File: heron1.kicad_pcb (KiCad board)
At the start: 2 copper layers, 38 parts, among them J1 7.4 V BAT, J2 Conn_02x11_Counter_Clockwise, J3 MotorA, J4 Motor B, SW1 SW_Wuerth_450301014042, U1 ESP32-S3-DevKitC, U2 L7805, U4 L7806, U6 VNH5019A-E, U7 VNH5019A-E

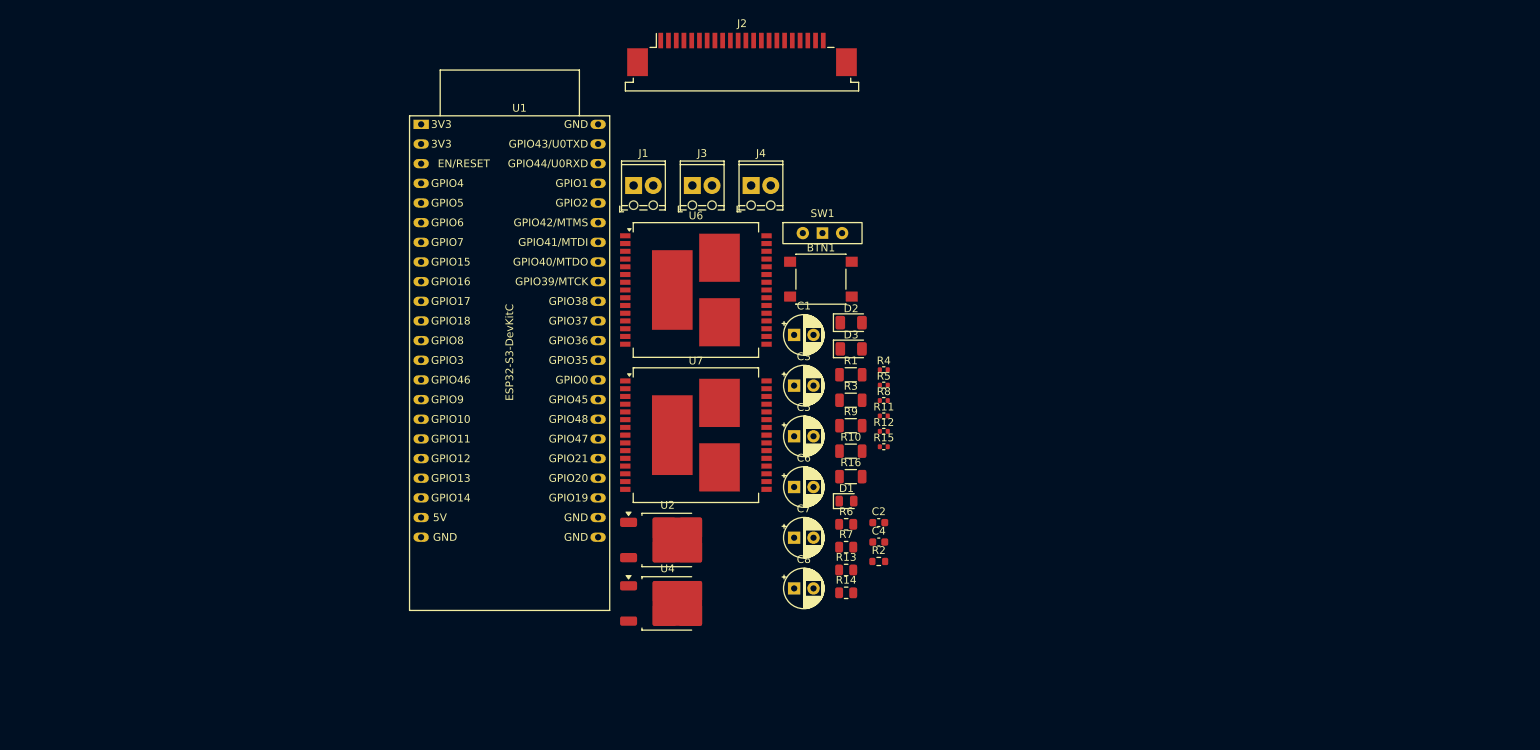
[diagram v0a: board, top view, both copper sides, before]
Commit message: first stage pcb
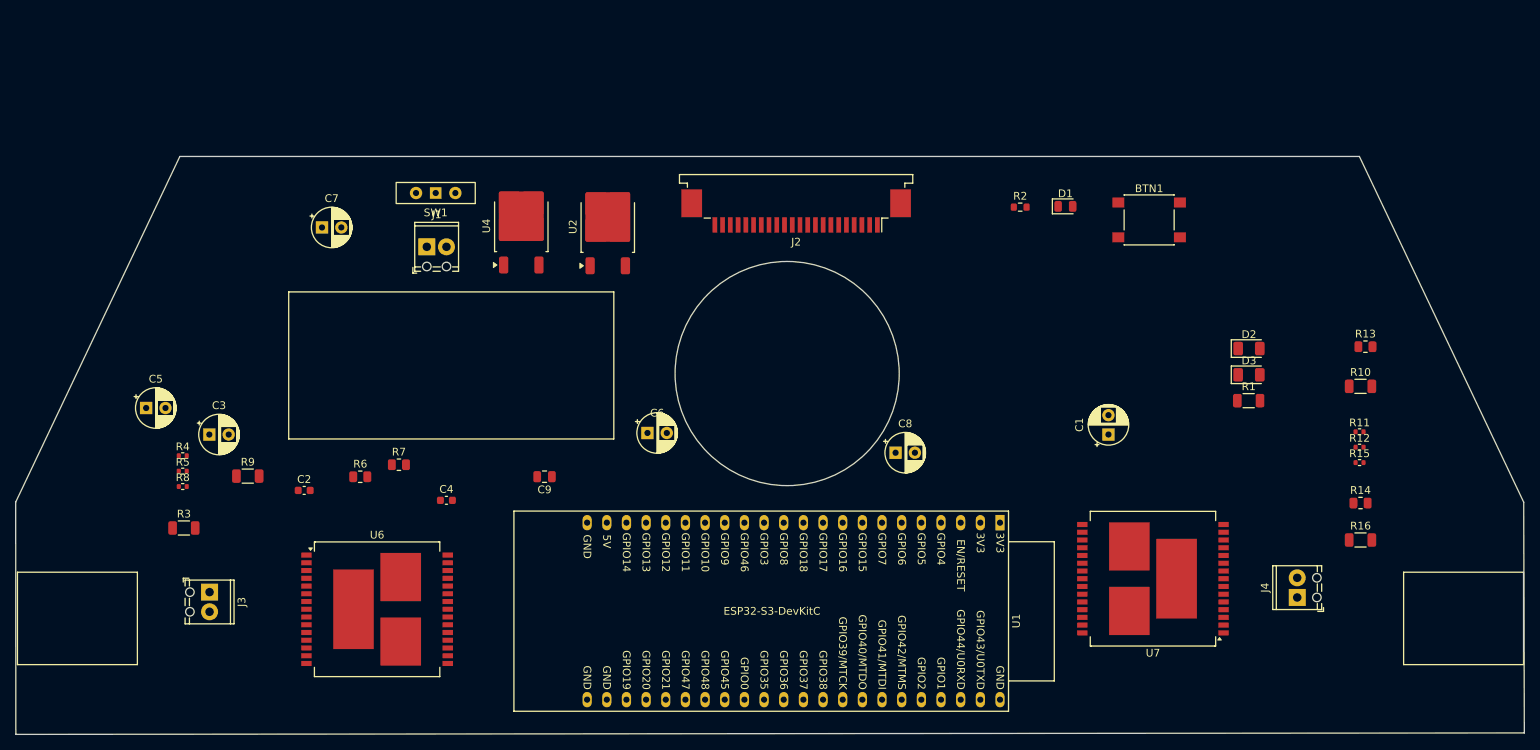
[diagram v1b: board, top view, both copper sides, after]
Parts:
- added C9: C, Capacitor_SMD:C_0805_2012Metric, F.Cu at (124.0, 92.0)
- moved R4 91.2 mm to (77.3, 89.3)
- moved R5 91.2 mm to (77.3, 91.3)
- moved R8 91.2 mm to (77.3, 93.3)
- moved U1 90.8 mm to (182.8, 98.0), turned to -90 degrees
- moved J4 88.4 mm to (221.2, 107.7), turned to 90 degrees
- moved R3 87.7 mm to (77.4, 98.7)
- moved C5 83.8 mm to (72.5, 83.2)
- moved J3 81.5 mm to (80.7, 107.0), turned to -90 degrees
- moved R9 78.2 mm to (85.7, 92.0)
- moved C3 75.8 mm to (80.7, 86.6)
- moved C2 74.3 mm to (93.0, 93.8)
- moved R13 73.0 mm to (230.1, 75.2)
- moved C7 73.0 mm to (95.2, 59.9)
- moved R14 67.5 mm to (229.4, 95.5)
- moved R10 66.4 mm to (229.4, 80.4)
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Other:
- board outline added: 194.9 x 74.7 mm
